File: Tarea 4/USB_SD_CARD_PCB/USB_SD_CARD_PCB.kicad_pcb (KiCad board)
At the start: 4 copper layers, 42.4 x 32.3 mm, 14 parts, among them J1 PZ254R-12-16P

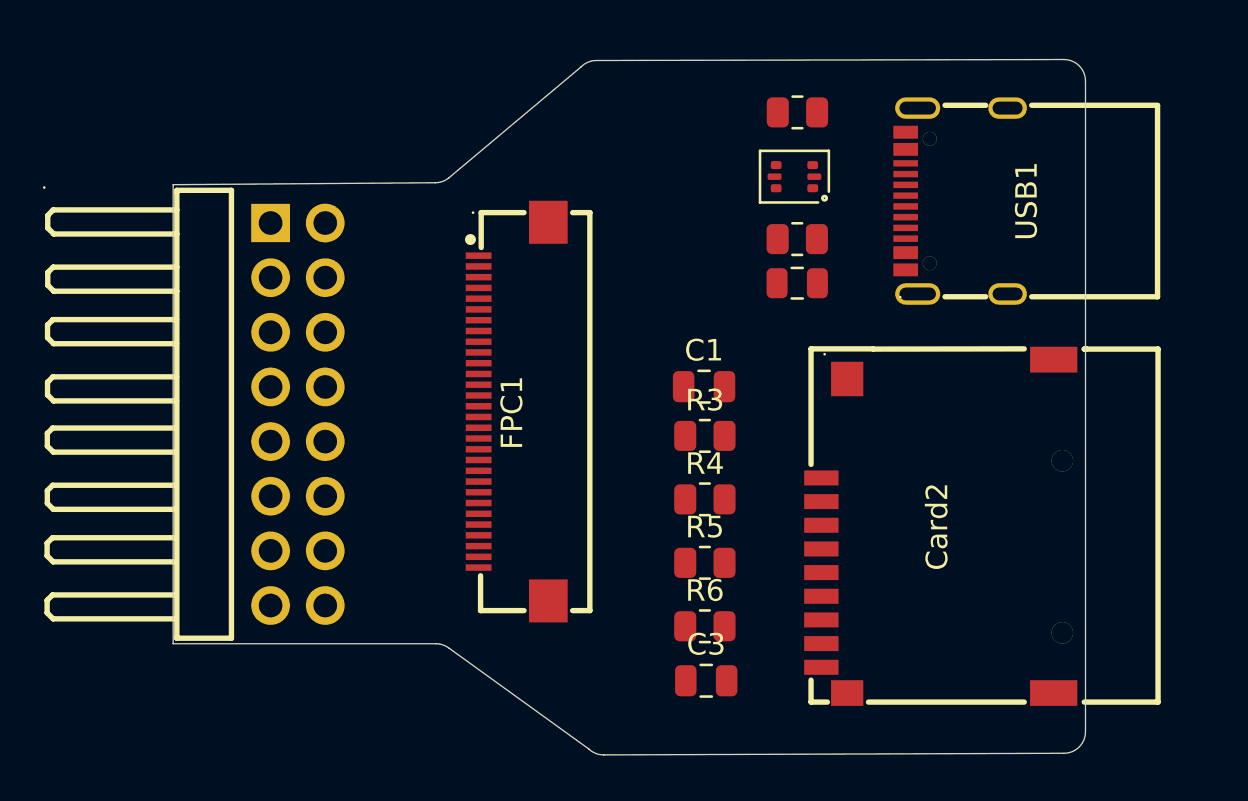
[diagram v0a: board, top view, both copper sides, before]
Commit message: Actualizacion 18/04/26
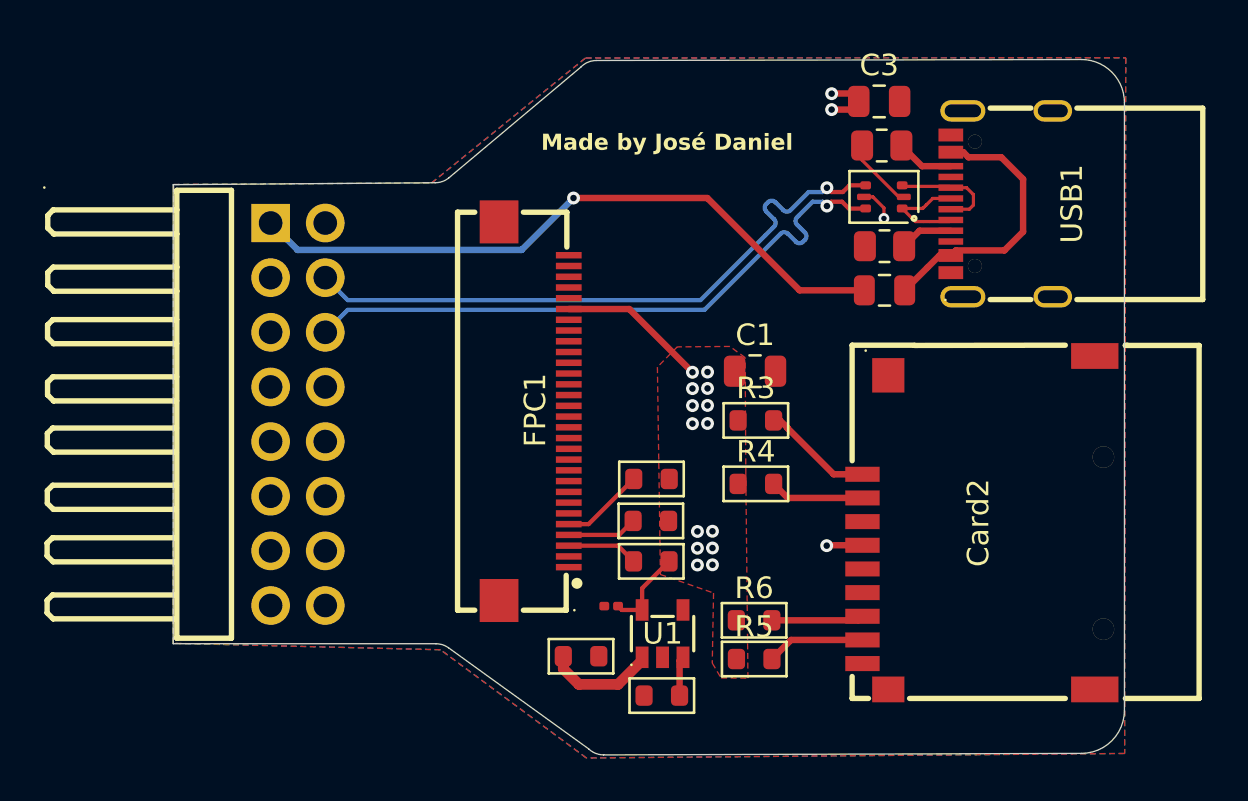
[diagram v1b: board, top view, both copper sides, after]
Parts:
- added C2: 10uF, Capacitor_SMD:C_0201_0603Metric, F.Cu at (113.6, 93.0)
- added R10: 10K, PCM_Resistor_SMD_AKL:R_0603_1608Metric, F.Cu at (115.5, 91.0)
- added R11: 10K, PCM_Resistor_SMD_AKL:R_0603_1608Metric, F.Cu at (115.5, 89.1)
- added R7: 6.8K, PCM_Resistor_SMD_AKL:R_0603_1608Metric, F.Cu at (116.0, 97.2)
- added R8: 300R, PCM_Resistor_SMD_AKL:R_0603_1608Metric, F.Cu at (112.2, 95.4)
- added R9: 10K, PCM_Resistor_SMD_AKL:R_0603_1608Metric, F.Cu at (115.5, 87.1)
- added U1: MT9700-N, EasyEDA:SOT-23-5_L2.9-W1.6-P0.95-LS2.9-BL, F.Cu at (116.0, 94.3)
- R3, R4, R5, R6: footprint Resistor_SMD:R_0805_2012Metric -> PCM_Resistor_SMD_AKL:R_0603_1608Metric
- moved C3 28.1 mm to (126.1, 69.6)
- moved R5 5.03 mm to (120.3, 95.5)
- moved D1 4.26 mm to (126.3, 74.0)
- moved R2 4.21 mm to (126.2, 71.6)
- moved F1 4.07 mm to (126.3, 78.4)
- moved R1 4.07 mm to (126.3, 76.3)
- moved C1 2.48 mm to (120.3, 82.1)
- moved R3 2.48 mm to (120.4, 84.4)
- moved R4 2.48 mm to (120.4, 87.4)
- moved R6 2.30 mm to (120.3, 93.7)
- moved USB1 2.10 mm to (131.8, 74.3)
- moved Card2 1.92 mm to (130.7, 89.2)
- moved FPC1 0.95 mm to (110.0, 84.0), turned to -90 degrees
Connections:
- FPC1 pad 1: unconnected-(FPC1-Pad1) -> GND
- FPC1 pad 2: unconnected-(FPC1-Pad2) -> VDD
- FPC1 pad 20: unconnected-(FPC1-Pad20) -> /LED+
- FPC1 pad 21: unconnected-(FPC1-Pad21) -> GND
- FPC1 pad 22: unconnected-(FPC1-Pad22) -> GND
- FPC1 pad 23: unconnected-(FPC1-Pad23) -> GND
- FPC1 pad 24: unconnected-(FPC1-Pad24) -> GND
- FPC1 pad 25: unconnected-(FPC1-Pad25) -> +3.3V
- FPC1 pad 26: unconnected-(FPC1-Pad26) -> /I2C_SCK
- FPC1 pad 27: unconnected-(FPC1-Pad27) -> /I2C_SDA
- FPC1 pad 28: unconnected-(FPC1-Pad28) -> /TP_INT
- FPC1 pad 29: unconnected-(FPC1-Pad29) -> /RESET
- FPC1 pad 3: unconnected-(FPC1-Pad3) -> /IM2
- FPC1 pad 30: unconnected-(FPC1-Pad30) -> GND
- FPC1 pad 31: unconnected-(FPC1-Pad31) -> GND
- FPC1 pad 32: unconnected-(FPC1-Pad32) -> GND
- FPC1 pad 4: unconnected-(FPC1-Pad4) -> /IM1
- FPC1 pad 5: unconnected-(FPC1-Pad5) -> /RESET
- FPC1 pad 6: unconnected-(FPC1-Pad6) -> /LCD_CS
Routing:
- net +5V: track 0.00 -> 30.9 mm, vias 0 -> 1
- net /USB-: track 0.00 -> 29.5 mm, vias 0 -> 1
- net /USB+: track 0.00 -> 29.5 mm, vias 0 -> 1
- net +3.3V: track 0.00 -> 17.1 mm, vias 0 -> 18
- net Net-(F1-Pad2): track 0.00 -> 13.0 mm
- net Net-(Card2-DAT2): track 0.00 -> 5.17 mm
- net VDD: track 0.00 -> 5.15 mm
- net /D+: track 0.00 -> 5.11 mm
- net /D-: track 0.00 -> 5.00 mm
- net Net-(Card2-DAT1): track 0.00 -> 4.58 mm
- net /SD_CS: track 0.00 -> 4.40 mm
- net /SPI_MISO: track 0.00 -> 4.29 mm
- net /RESET: track 0.00 -> 3.89 mm
- net GND: track 0.00 -> 3.33 mm
- net /IM2: track 0.00 -> 3.31 mm
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- added copper zone on B.Cu, net +3.3V
- added copper zone on F.Cu, net +3.3V
- added copper zone on F.Cu, net GND
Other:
- board size 42.4 x 32.3 mm -> 44.2 x 32.3 mm
- board text added: "Made by José Daniel"
